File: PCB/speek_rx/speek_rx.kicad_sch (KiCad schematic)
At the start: 61 parts, among them CN1 PJ-320D, J1 Conn_01x02, SW1 TS-1187A-B-A-B, SW2 TS-1187A-B-A-B, U1 ESP32-D0WD-V3, U2 W25Q32JVSSIQ_C179173, U3 CP2102N-A02-GQFN24R, U4 SPX1117M3-L-3-3/TR, U5 PCM5102APW, U6 TPA6132A2RTER, X1 XL2EL89CPI-111YLC-40M

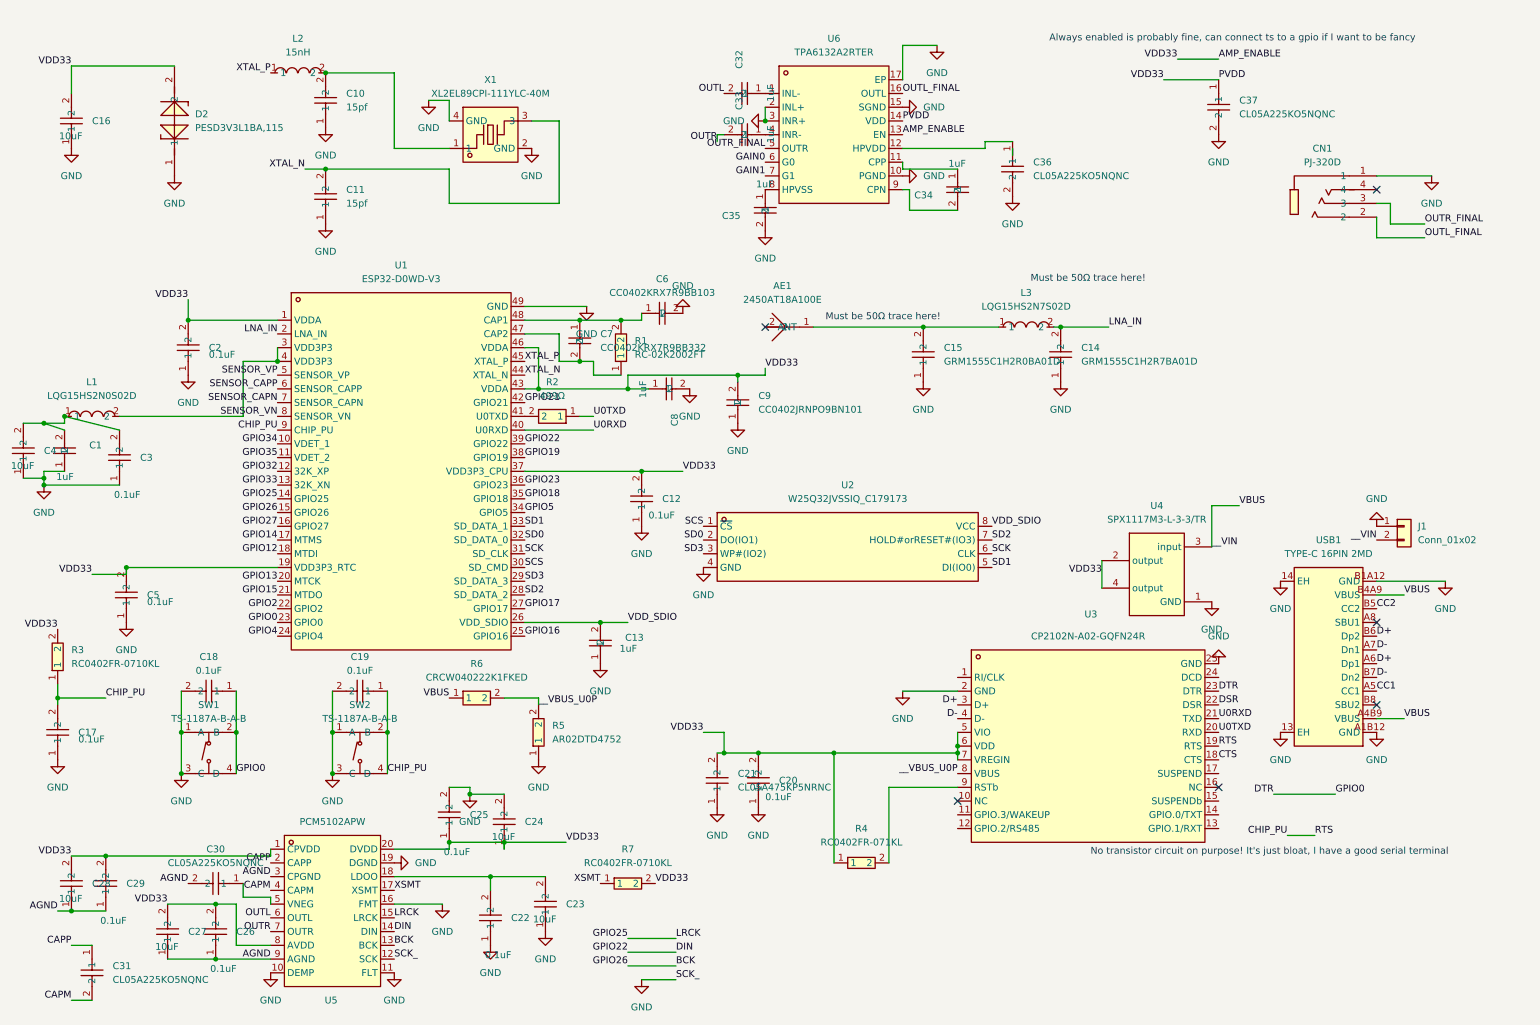
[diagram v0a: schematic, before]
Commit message: easy layout done
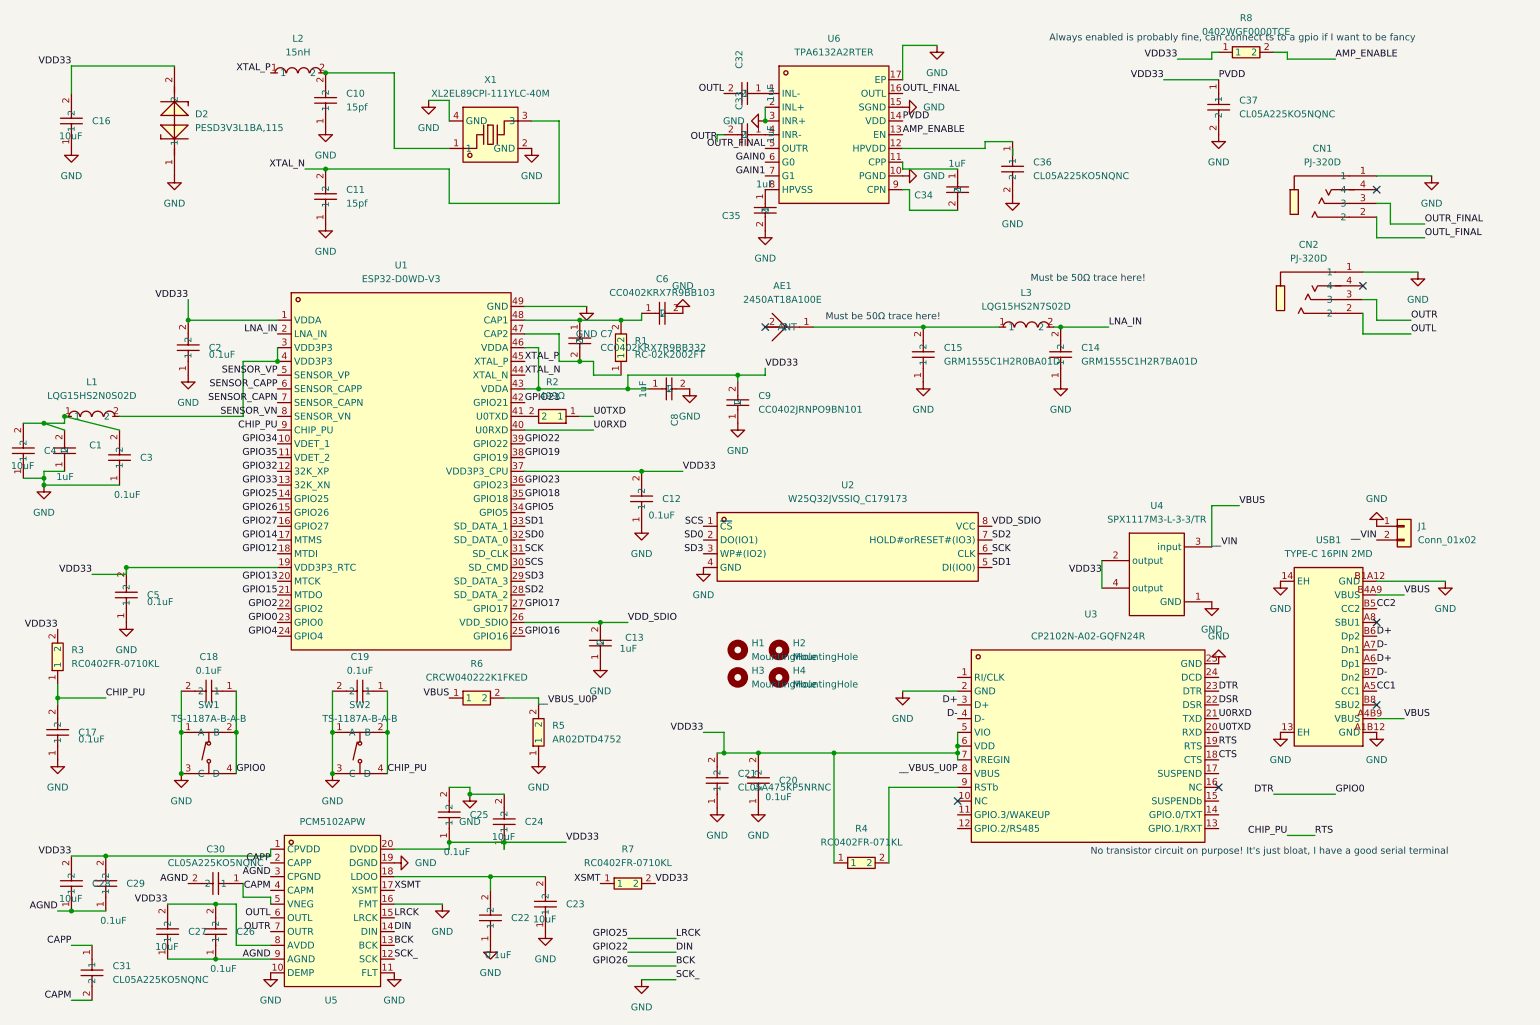
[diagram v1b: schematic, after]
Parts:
- added CN2: PJ-320D, easyeda2kicad:AUDIO-SMD_PJ-320D-1, symbol lcsc:PJ-320D
- added H1, H2, H3, H4: MountingHole, MountingHole:MountingHole_3.2mm_M3, symbol Mechanical:MountingHole
- added R8: 0402WGF0000TCE, easyeda2kicad:R0402, symbol lcsc:0402WGF0000TCE
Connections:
- net AMP_ENABLE: now also R8.2; no longer C12.2, C16.2, C2.2, C20.2, C21.2, C24.1, C25.1, C26.2, C27.2, C28.2, C29.2, C37.1, C5.2, C8.1, C9.2, D2.2, R3.2, R4.1, R7.2, U1.1 (VDDA), U1.19 (VDD3P3_RTC), U1.37 (VDD3P3_CPU), U1.43 (VDDA), U1.46 (VDDA), U3.5 (VIO), U3.6 (VDD), U3.7 (VREGIN), U4.2 (output), U4.4 (output), U5.1 (CPVDD), U5.20 (DVDD), U5.8 (AVDD), U6.14 (VDD)
- net GND: now also CN2.1
- net OUTL: now also CN2.2
- net OUTR: now also CN2.3
- new net PVDD: C12.2, C16.2, C2.2, C20.2, C21.2, C24.1, C25.1, C26.2, C27.2, C28.2, C29.2, C37.1, C5.2, C8.1, C9.2, D2.2, R3.2, R4.1, R7.2, R8.1, U1.1 (VDDA), U1.19 (VDD3P3_RTC), U1.37 (VDD3P3_CPU), U1.43 (VDDA), U1.46 (VDDA), U3.5 (VIO), U3.6 (VDD), U3.7 (VREGIN), U4.2 (output), U4.4 (output), U5.1 (CPVDD), U5.20 (DVDD), U5.8 (AVDD), U6.14 (VDD)
- no-connect marks 6 -> 7
